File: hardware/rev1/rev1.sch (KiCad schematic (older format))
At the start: 37 parts, among them J1 Conn_01x09_Male, J2 Conn_01x09_Male, J3 Conn_01x09_Male, U1 BNO055, U2 MPL3115A2, U3 Teensy3.6, U4 BMI088, U5 ADXL345BCCZ, Y1 Crystal_32kHz768

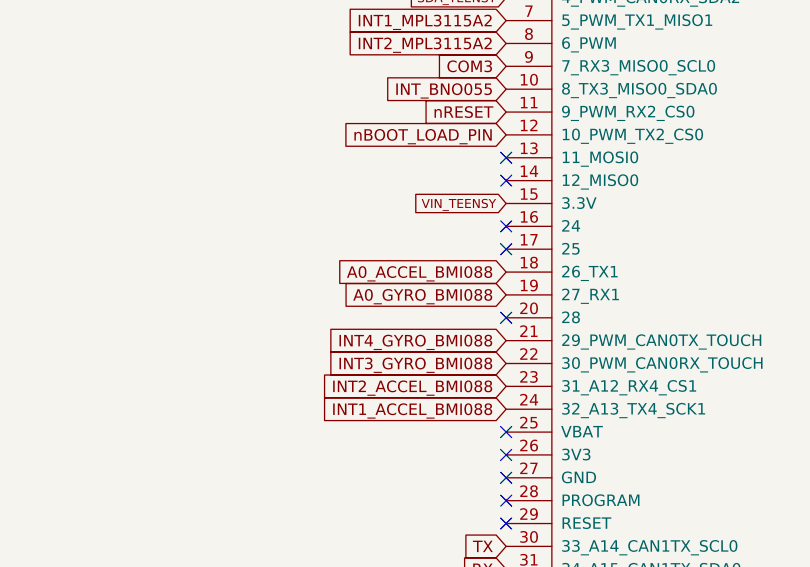
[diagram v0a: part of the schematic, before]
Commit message: wip
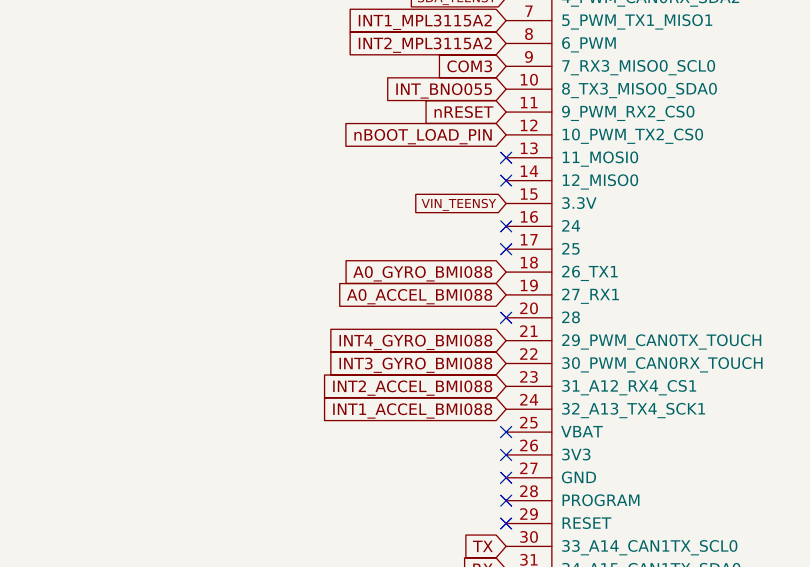
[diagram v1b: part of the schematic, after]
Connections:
- net A0_ACCEL_BMI088: now also U3.19 (27_RX1); no longer U3.18 (26_TX1)
- net A0_GYRO_BMI088: now also U3.18 (26_TX1); no longer U3.19 (27_RX1)
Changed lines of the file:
@@
 Text GLabel 27400 4800 0    50   Input ~ 0
 INT4_GYRO_BMI088
+Text GLabel 27400 4500 0    50   Input ~ 0
+A0_GYRO_BMI088
 Text GLabel 27400 4600 0    50   Input ~ 0
-A0_GYRO_BMI088
-Text GLabel 27400 4500 0    50   Input ~ 0
 A0_ACCEL_BMI088
 Text GLabel 27400 5800 0    50   Input ~ 0
